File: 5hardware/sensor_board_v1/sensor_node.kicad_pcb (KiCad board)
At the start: 2 copper layers, 24.2 x 24.2 mm, 31 parts, among them J1 Conn_01x09_Pin, Q2 AO3401A, Q3 AO3400A, SW1 SW_Push, SW2 SW_Push, U12 APDS-9960, U13 SHT31-DIS, U17 BH1750FVI-TR, U3 INA219AxDCN, U4 2N7002DW, U7 XC6206PxxxMR, U8 TPL5110

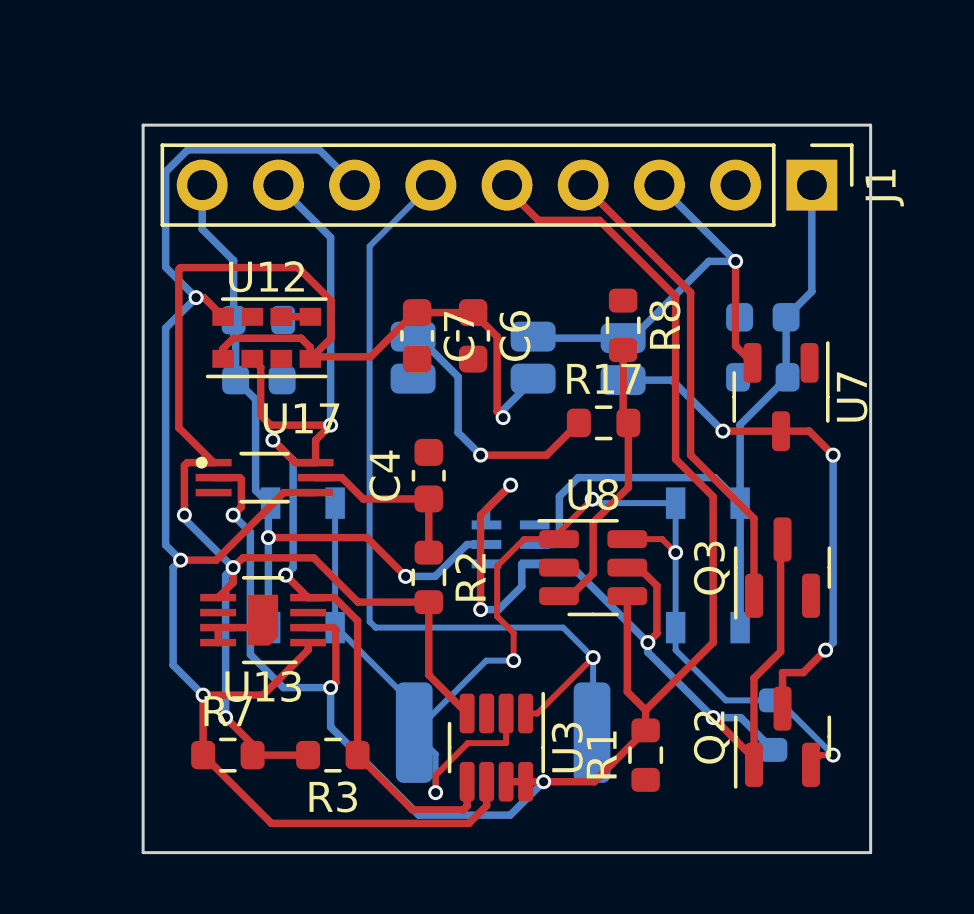
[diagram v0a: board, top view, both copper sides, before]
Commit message: update pcb.
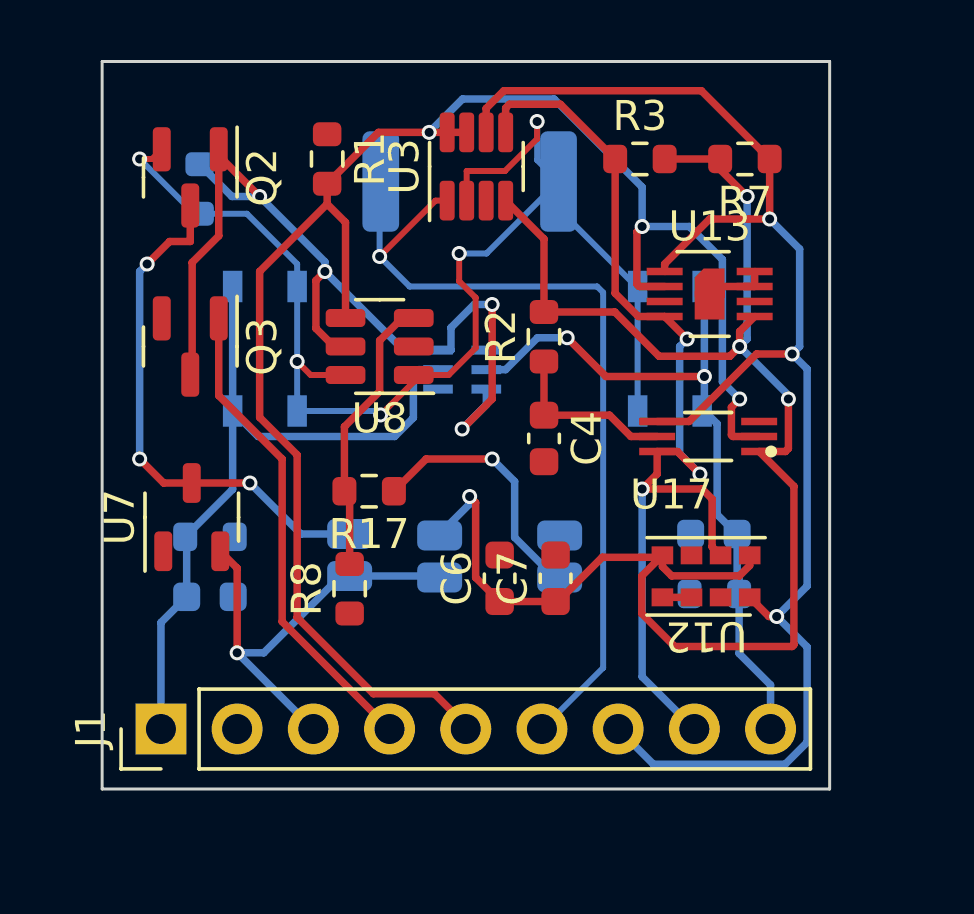
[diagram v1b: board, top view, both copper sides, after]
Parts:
- moved J1 28.3 mm to (90.3, 86.9), turned to 90 degrees
- moved Q2 27.2 mm to (91.3, 68.5), turned to -90 degrees
- moved R7 26.3 mm to (109.8, 67.9), turned to 180 degrees
- moved R19 26.2 mm to (91.6, 68.9), turned to -90 degrees
- moved R1 22.5 mm to (95.9, 67.9), turned to -90 degrees
- moved R3 22.4 mm to (106.3, 67.9), turned to 0 degrees
- moved Q3 21.1 mm to (91.3, 74.1), turned to -90 degrees
- moved C8 20.7 mm to (92.0, 82.5), turned to 0 degrees
- moved U7 20.0 mm to (91.4, 79.8), turned to 90 degrees
- moved U3 19.4 mm to (100.9, 68.1), turned to 90 degrees
- moved R16 19.2 mm to (92.0, 80.5), turned to 180 degrees
- moved U13 18.4 mm to (108.6, 72.4), turned to 0 degrees
- moved R15 18.4 mm to (100.6, 68.6), turned to 180 degrees
- moved R11 17.7 mm to (108.8, 82.4), turned to 0 degrees
- moved U12 16.7 mm to (108.5, 81.8), turned to 180 degrees
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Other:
- board size 24.2 x 24.2 mm -> 24.2 x 24.3 mm
